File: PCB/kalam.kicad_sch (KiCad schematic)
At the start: 17 parts, among them J1 Conn_01x04, J2 Conn_01x04, SW1 SW_Push, SW2 SW_Push, U1 XC6206PxxxMR, U2 STM32F072CBTx

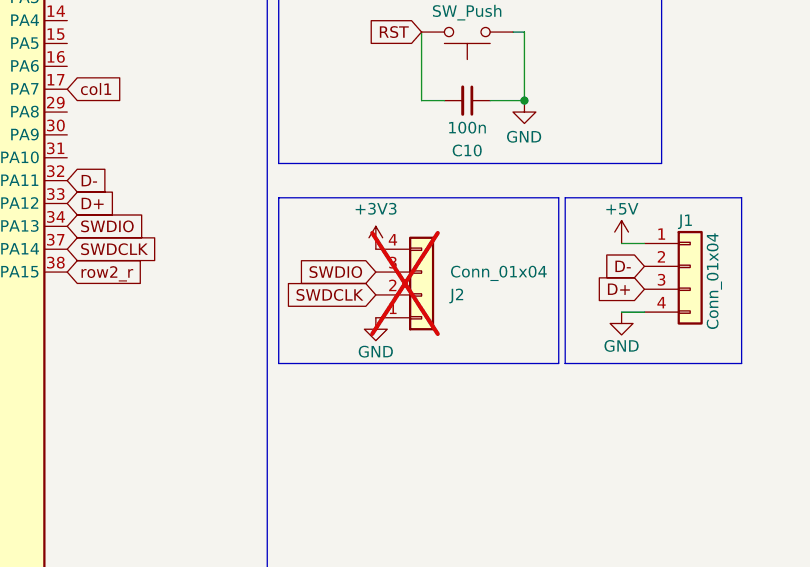
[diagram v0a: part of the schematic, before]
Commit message: PCB Fab v1
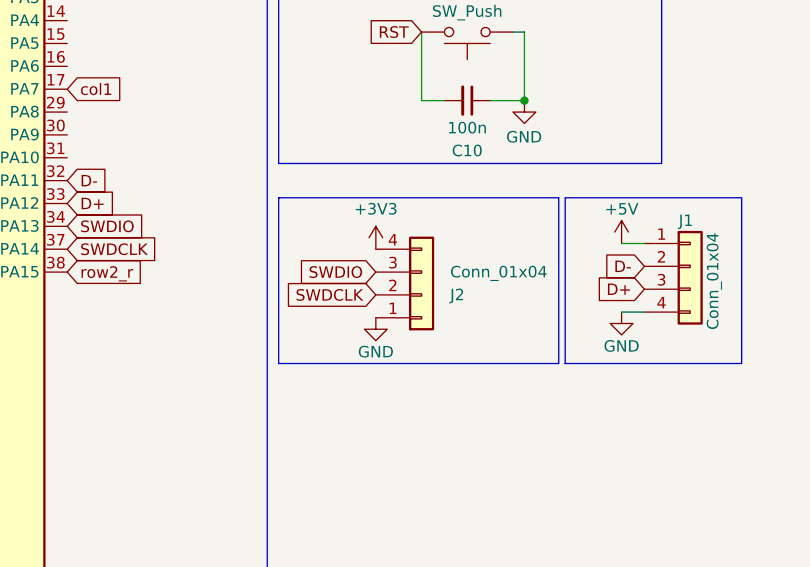
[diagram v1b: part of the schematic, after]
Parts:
- C1, C10, C2, C4: LCSC C1525 -> (none)
- C3, C5: LCSC C19666 -> (none)
- C6: LCSC C15195 -> (none)
- C7, C8, C9: LCSC C52923 -> (none)
- J1: LCSC C160404 -> (none)
- J2: now fitted
- R1: LCSC C25744 -> (none)
- SW1, SW2: LCSC C318884 -> (none)
- U1: LCSC C5148692 -> (none)
- U2: LCSC C81720 -> (none)
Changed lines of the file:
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@@
-			)
-		)
-		(property "LCSC" "C318884"
-			(at 110.49 24.13 0)
-			(effects
-				(font
-					(size 1.27 1.27)
-				)
-				(hide yes)
 			)
 		)
@@
 			)
 		)
-		(property "LCSC" "C318884"
-			(at 110.49 66.04 0)
-			(effects
-				(font
-					(size 1.27 1.27)
-				)
-				(hide yes)
-			)
-		)
 		(pin "1"
 		)
@@
 		)
 		(property "Description" ""
-			(at 135.255 92.075 0)
-			(effects
-				(font
-					(size 1.27 1.27)
-				)
-				(hide yes)
-			)
-		)
-		(property "LCSC" "C160404"
 			(at 135.255 92.075 0)
 			(effects
@@
 			)
 		)
-		(property "LCSC" "C25744"
-			(at 118.11 26.67 0)
-			(effects
-				(font
-					(size 1.27 1.27)
-				)
-				(hide yes)
-			)
-		)
 		(pin "1"
 		)
@@
 			)
 		)
-		(property "LCSC" "C19666"
-			(at 45.085 24.13 0)
-			(effects
-				(font
-					(size 1.27 1.27)
-				)
-				(hide yes)
-			)
-		)
 		(pin "1"
 		)
@@
 			)
 		)
-		(property "LCSC" "C1525"
-			(at 36.83 24.13 0)
-			(effects
-				(font
-					(size 1.27 1.27)
-				)
-				(hide yes)
-			)
-		)
 		(pin "1"
 		)
@@
 			)
 		)
-		(property "LCSC" "C1525"
-			(at 28.575 24.13 0)
-			(effects
-				(font
-					(size 1.27 1.27)
-				)
-				(hide yes)
-			)
-		)
 		(pin "1"
 		)
@@
 			)
 		)
-		(property "LCSC" "C1525"
-			(at 36.83 35.56 0)
-			(effects
-				(font
-					(size 1.27 1.27)
-				)
-				(hide yes)
-			)
-		)
 		(pin "1"
 		)
@@
 		)
 		(property "Description" ""
-			(at 123.19 46.99 0)
-			(effects
-				(font
-					(size 1.27 1.27)
-				)
-				(hide yes)
-			)
-		)
-		(property "LCSC" "C52923"
 			(at 123.19 46.99 0)
 			(effects
@@
 			)
 		)
-		(property "LCSC" "C52923"
-			(at 66.675 37.465 0)
-			(effects
-				(font
-					(size 1.27 1.27)
-				)
-				(hide yes)
-			)
-		)
 		(pin "1"
 		)
@@
 			)
 		)
-		(property "LCSC" "C5148692"
-			(at 110.49 44.45 0)
-			(effects
-				(font
-					(size 1.27 1.27)
-				)
-				(hide yes)
-			)
-		)
 		(pin "1"
 		)
@@
 		)
 		(property "Description" ""
-			(at 58.42 37.465 0)
-			(effects
-				(font
-					(size 1.27 1.27)
-				)
-				(hide yes)
-			)
-		)
-		(property "LCSC" "C15195"
 			(at 58.42 37.465 0)
 			(effects
@@
 			)
 		)
-		(property "LCSC" "C1525"
-			(at 110.49 73.66 0)
-			(effects
-				(font
-					(size 1.27 1.27)
-				)
-				(hide yes)
-			)
-		)
 		(pin "1"
 		)
@@
 		(in_bom yes)
 		(on_board yes)
-		(dnp yes)
+		(dnp no)
 		(property "Reference" "J2"
 			(at 108.585 95.25 0)
@@
 			)
 		)
-		(property "LCSC" "C81720"
-			(at 48.26 90.17 0)
-			(effects
-				(font
-					(size 1.27 1.27)
-				)
-				(hide yes)
-			)
-		)
 		(pin "23"
 		)
@@
 			)
 		)
-		(property "LCSC" "C52923"
-			(at 97.79 46.99 0)
-			(effects
-				(font
-					(size 1.27 1.27)
-				)
-				(hide yes)
-			)
-		)
 		(pin "1"
 		)
@@
 			(at 45.085 35.56 0)
 			(effects
-				(font
-					(size 1.27 1.27)
-				)
-				(hide yes)
-			)
-		)
-		(property "LCSC" "C19666"
-			(at 45.085 35.56 0)
-			(effects

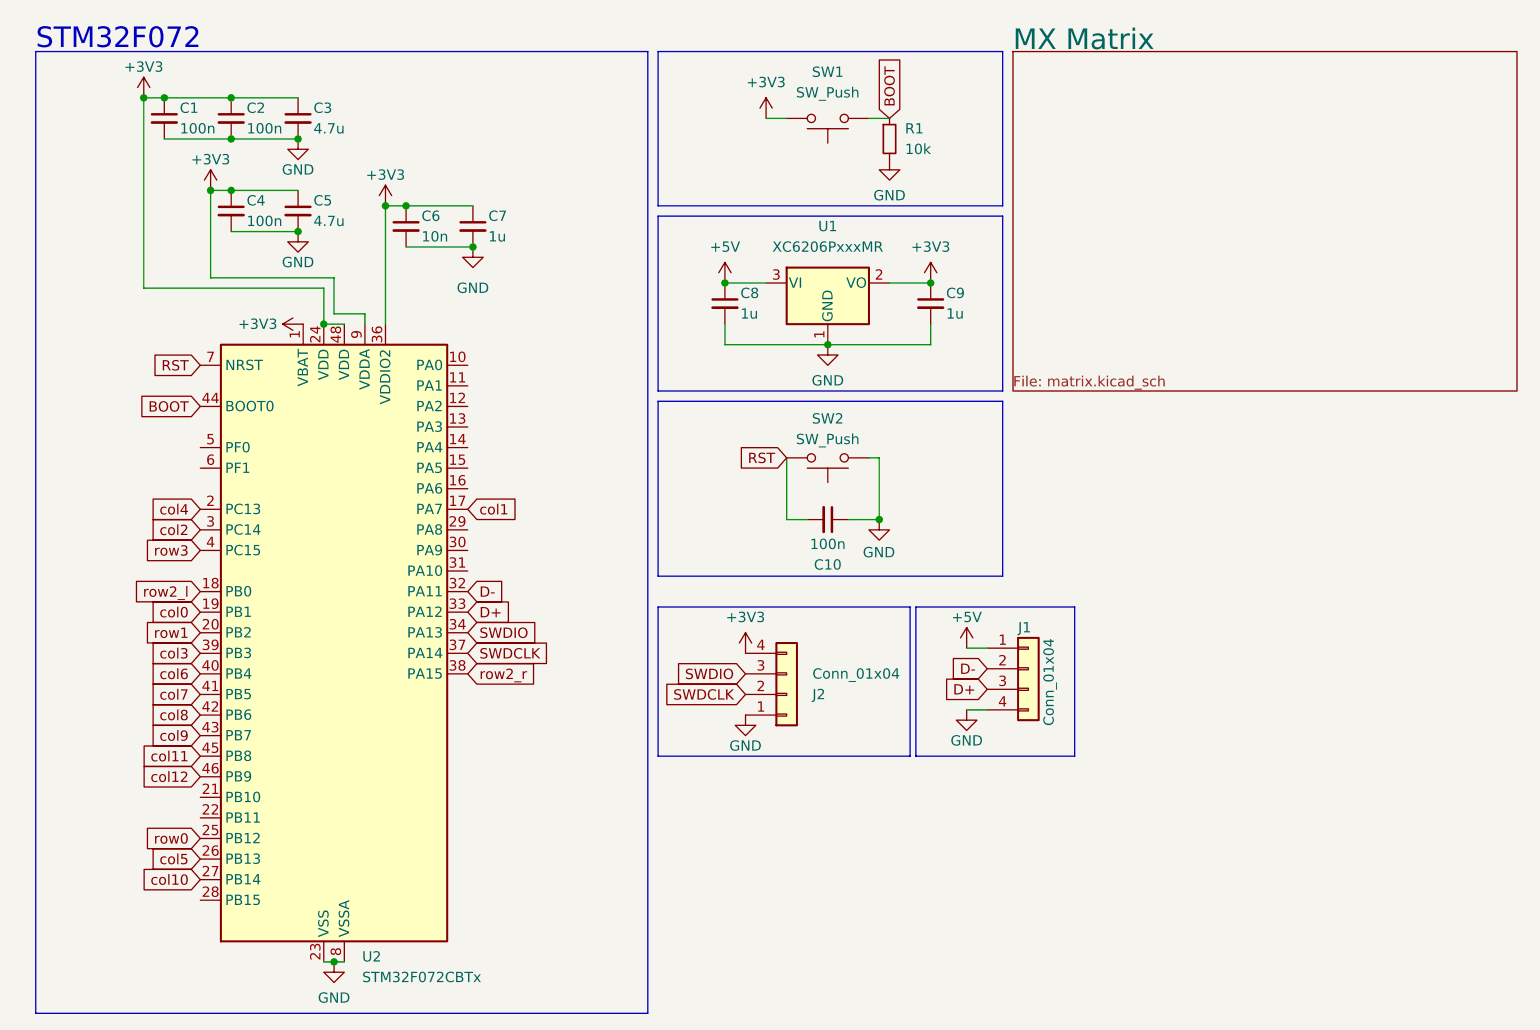
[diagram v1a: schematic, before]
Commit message: updates
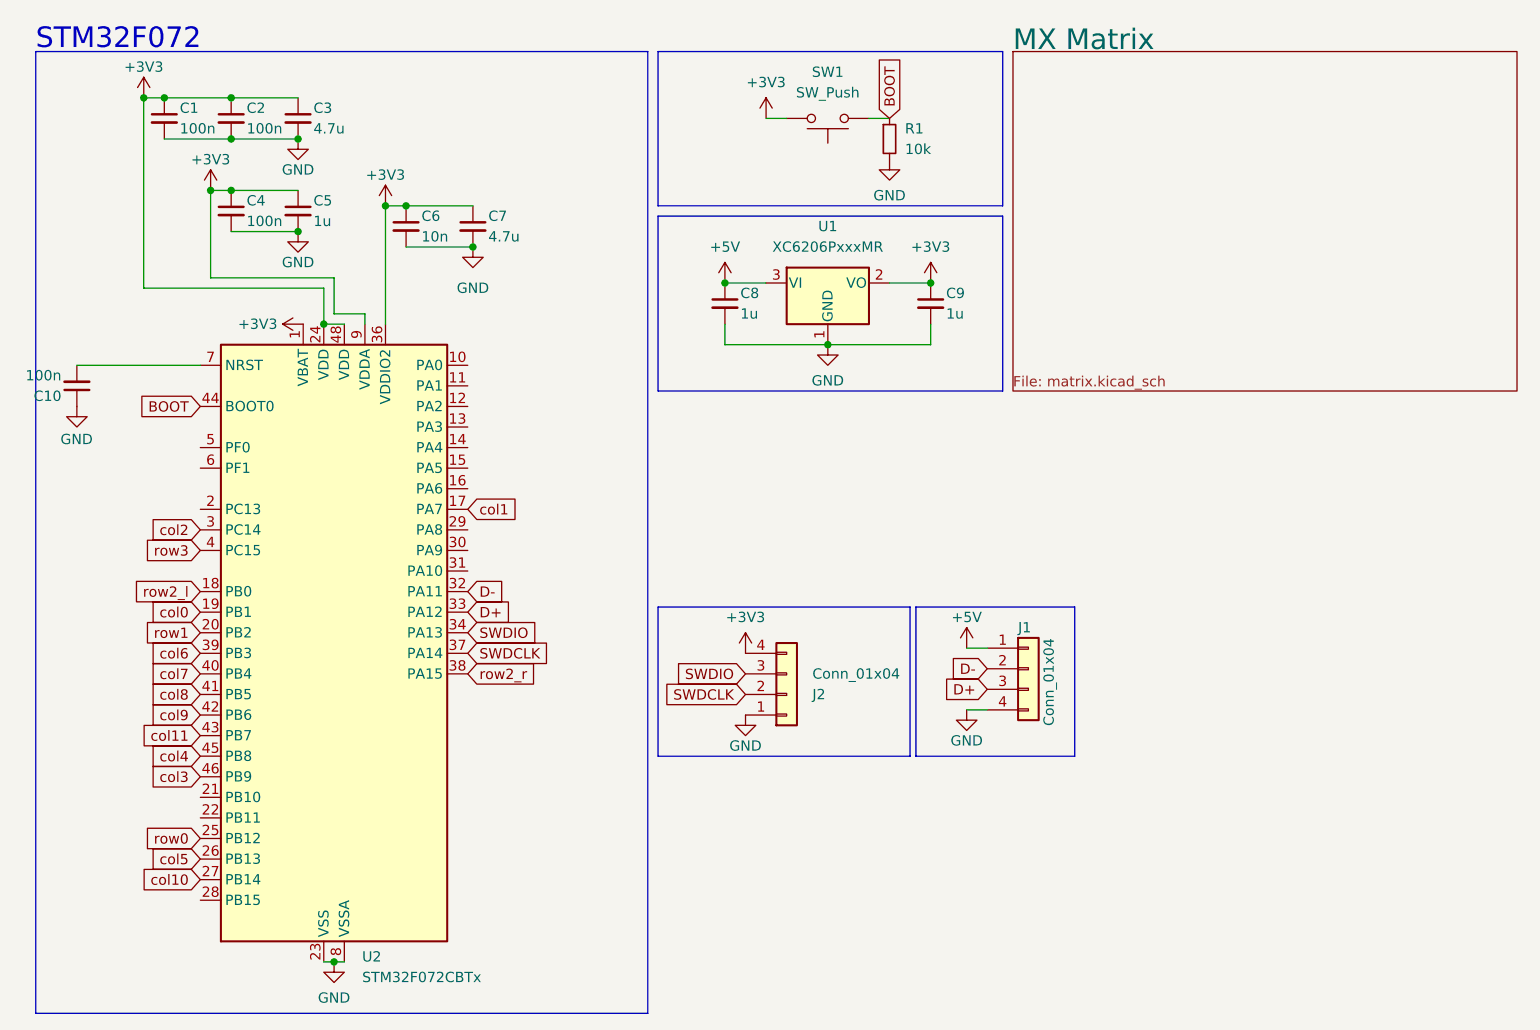
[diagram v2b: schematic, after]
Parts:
- removed SW2: SW_Push, Button_Switch_SMD:SW_Push_1P1T_XKB_TS-1187A, symbol Switch:SW_Push
- C5: value 4.7u -> 1u
- C7: value 1u -> 4.7u
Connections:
- net col12 is gone; now on net col3: U2.46 (PB9)
- net col11: now also U2.43 (PB7); no longer U2.45 (PB8)
- net col3: no longer U2.39 (PB3)
- net col4: now also U2.45 (PB8); no longer U2.2 (PC13)
- net col6: now also U2.39 (PB3); no longer U2.40 (PB4)
- net col7: now also U2.40 (PB4); no longer U2.41 (PB5)
- net col8: now also U2.41 (PB5); no longer U2.42 (PB6)
- net col9: now also U2.42 (PB6); no longer U2.43 (PB7)
- net RST: no longer names the net of C10.2, U2.7 (NRST)

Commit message: back to the drawing board
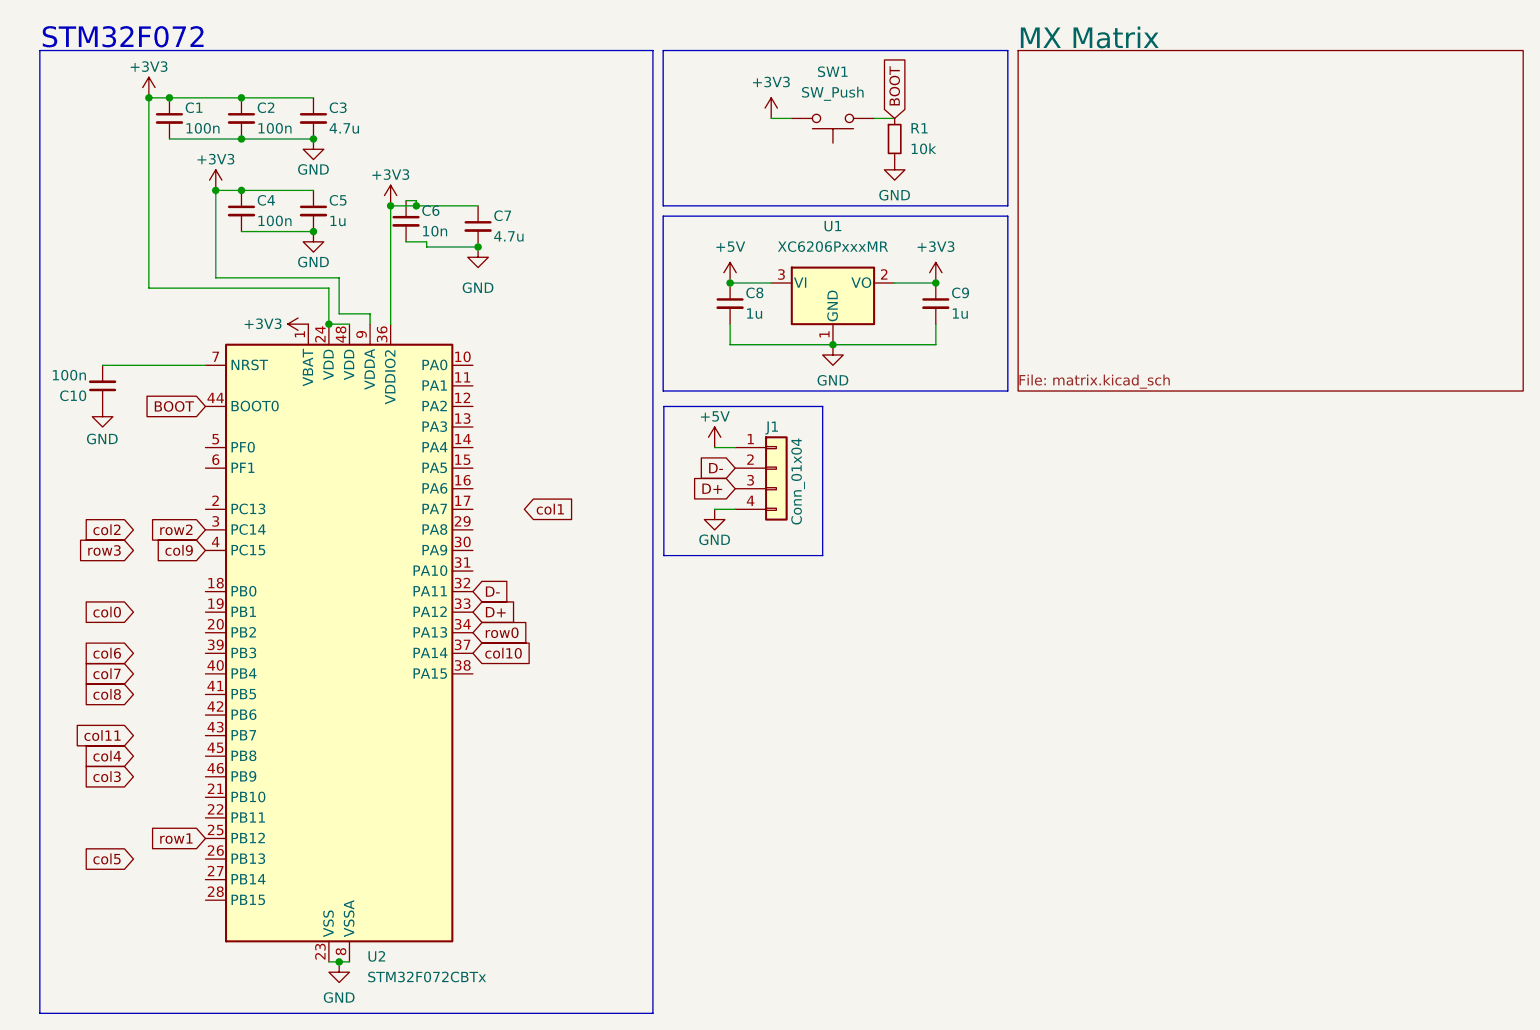
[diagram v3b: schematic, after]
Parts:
- removed J2: Conn_01x04, Connector_PinHeader_2.54mm:PinHeader_1x04_P2.54mm_Vertical, symbol Connector_Generic:Conn_01x04
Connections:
- net SWDCLK is gone; now on net col10: U2.37 (PA14)
- net SWDIO is gone; now on net row0: U2.34 (PA13)
- net col0: no longer U2.19 (PB1)
- net col1: no longer U2.17 (PA7)
- net col10: no longer U2.27 (PB14)
- net col11: no longer U2.43 (PB7)
- net col2: no longer U2.3 (PC14)
- net col3: no longer U2.46 (PB9)
- net col4: no longer U2.45 (PB8)
- net col5: no longer U2.26 (PB13)
- net col6: no longer U2.39 (PB3)
- net col7: no longer U2.40 (PB4)
- net col8: no longer U2.41 (PB5)
- net col9: now also U2.4 (PC15); no longer U2.42 (PB6)
- net row0: no longer U2.25 (PB12)
- net row1: now also U2.25 (PB12); no longer U2.20 (PB2)
- net row3: no longer U2.4 (PC15)
- net row2_l: no longer names the net of U2.18 (PB0)
- net row2_r: no longer names the net of U2.38 (PA15)
- new net row2: U2.3 (PC14)
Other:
- moved on the sheet: C1, C10, C2, C4, C5, C6, C7, C8, C9, J1, R1, SW1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

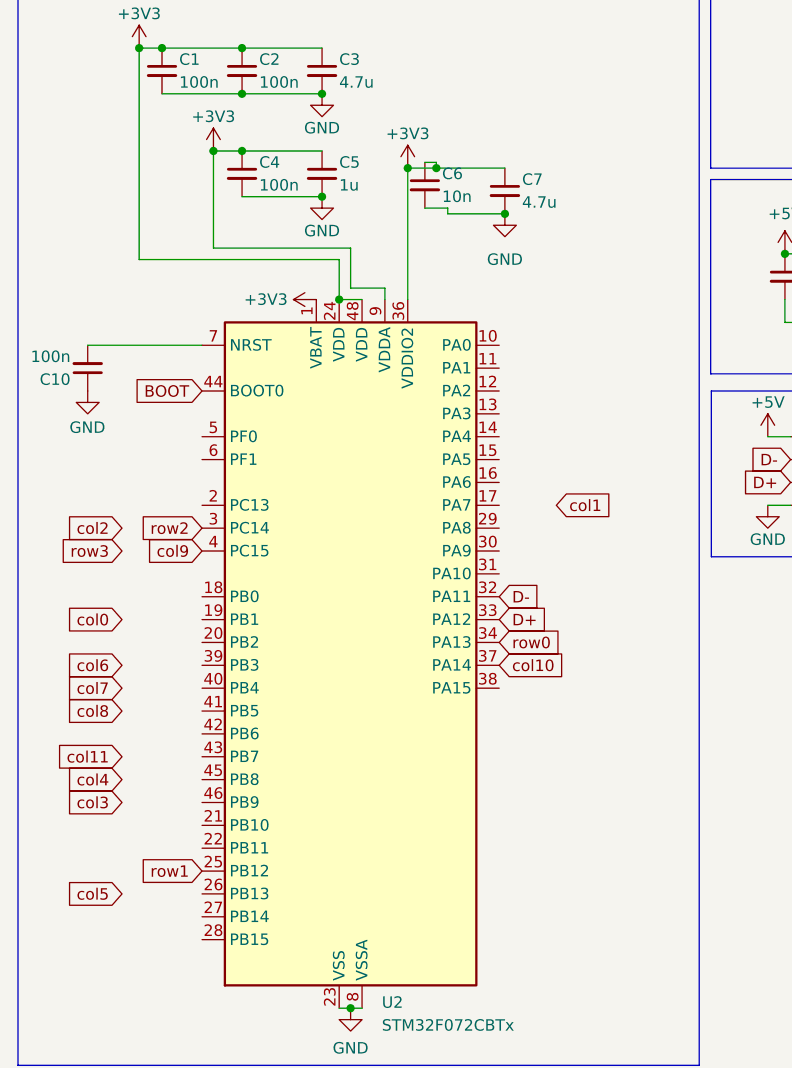
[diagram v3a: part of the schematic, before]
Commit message: beeg overhaul and new layout image
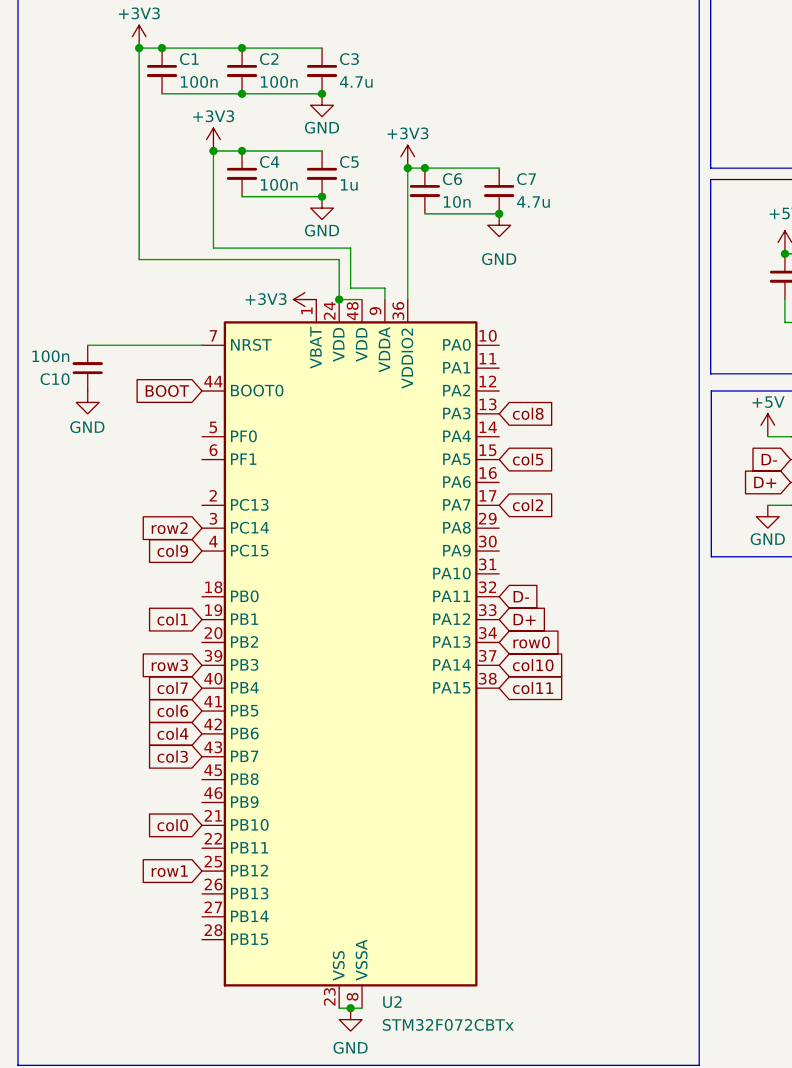
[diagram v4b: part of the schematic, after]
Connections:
- net col0: now also U2.21 (PB10)
- net col1: now also U2.19 (PB1)
- net col11: now also U2.38 (PA15)
- net col2: now also U2.17 (PA7)
- net col3: now also U2.43 (PB7)
- net col4: now also U2.42 (PB6)
- net col5: now also U2.15 (PA5)
- net col6: now also U2.41 (PB5)
- net col7: now also U2.40 (PB4)
- net col8: now also U2.13 (PA3)
- net row3: now also U2.39 (PB3)
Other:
- moved on the sheet: C6, C7
